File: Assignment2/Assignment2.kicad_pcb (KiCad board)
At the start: 2 copper layers, 51 parts, among them J1 USB_B_Micro, J2 Conn_01x02, J3 Conn_01x03, J4 Conn_01x02, SW1 SW_Push, U1 RP2040, U2 NCP1117-3.3_SOT223, U3 W25Q128JVS, U4 ABM8-272-T3, U5 MAX98357A, U6 VEML6040

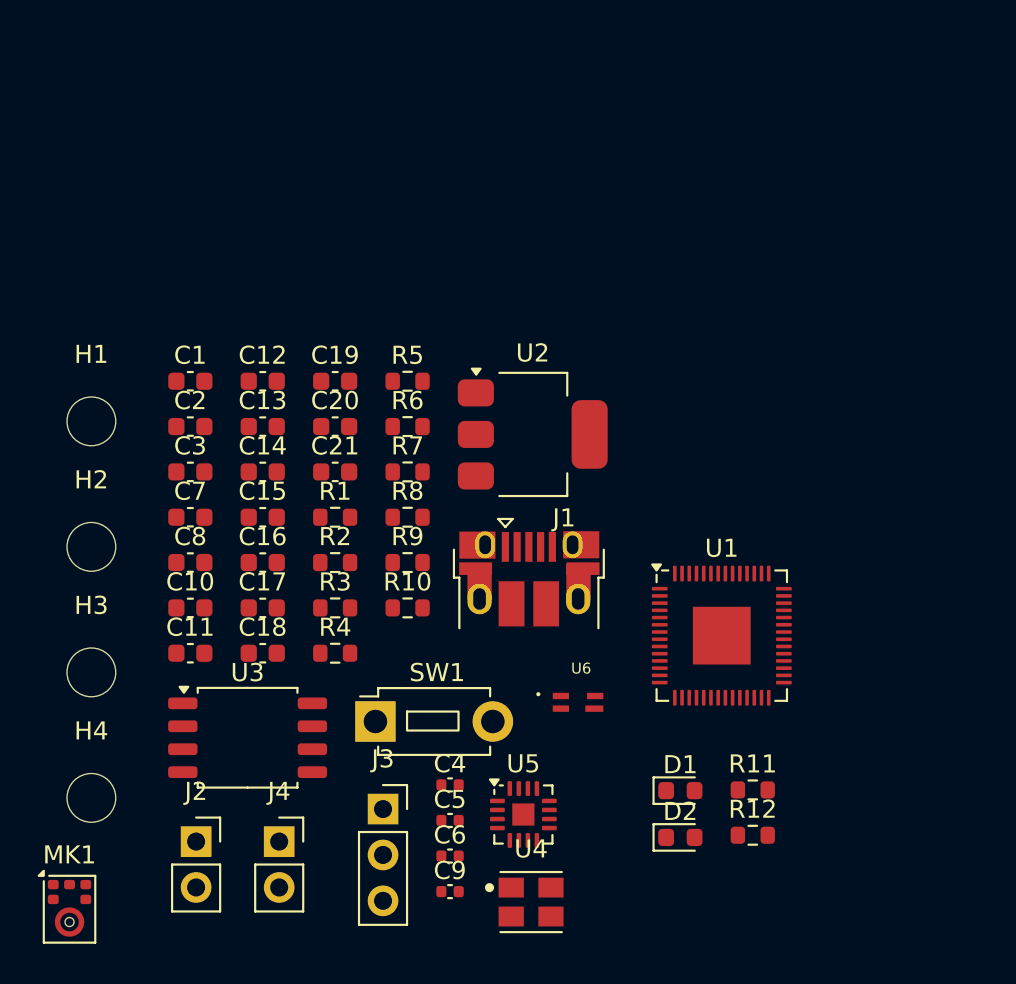
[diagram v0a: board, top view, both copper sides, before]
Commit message: route
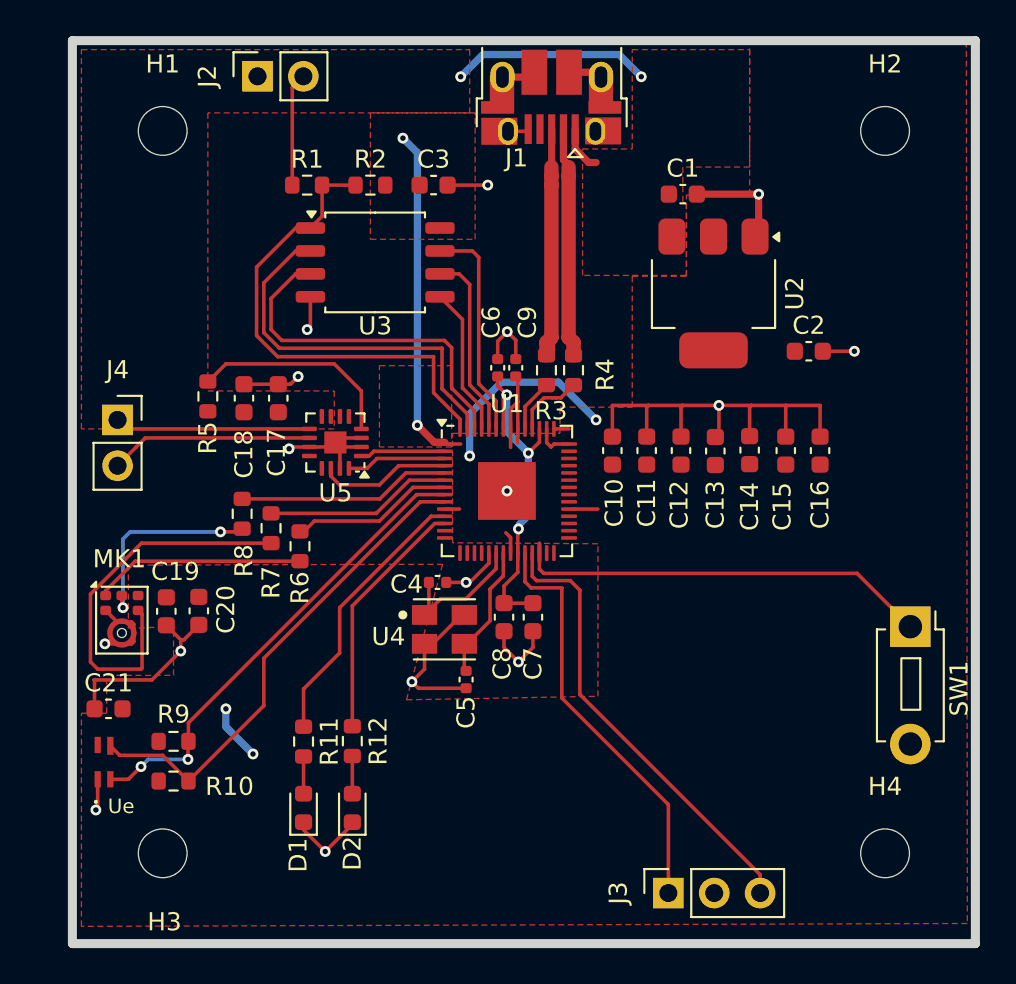
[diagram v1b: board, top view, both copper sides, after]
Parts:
- moved H2 49.6 mm to (145.0, 55.0)
- moved H4 44.1 mm to (145.0, 95.0)
- moved J2 42.5 mm to (110.2, 52.0), turned to 90 degrees
- moved C2 34.5 mm to (140.8, 67.2)
- moved C16 31.5 mm to (141.4, 72.7), turned to 90 degrees
- moved SW1 30.1 mm to (146.4, 82.5), turned to -90 degrees
- moved C9 29.2 mm to (124.5, 68.1), turned to 90 degrees
- moved C15 29.2 mm to (139.5, 72.7), turned to 90 degrees
- moved C1 29.2 mm to (133.8, 58.5)
- moved C11 27.6 mm to (131.8, 72.7), turned to 90 degrees
- moved U3 27.3 mm to (116.8, 62.3)
- moved C6 27.2 mm to (123.5, 68.1), turned to 90 degrees
- moved C14 27.0 mm to (137.5, 72.7), turned to 90 degrees
- moved J1 26.7 mm to (126.5, 53.1), turned to 180 degrees
- moved Ue 26.5 mm to (101.8, 90.0), turned to 90 degrees
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- renumbered U6 to Ue
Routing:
- net GND: track 0.00 -> 92.3 mm, vias 0 -> 16
- net +3.3V: track 0.00 -> 46.0 mm, vias 0 -> 6
- net /GPIO7: track 0.00 -> 27.3 mm
- net /QSPI_SS: track 0.00 -> 27.1 mm
- net /GPIO6: track 0.00 -> 26.2 mm, vias 0 -> 2
- net /SWD: track 0.00 -> 25.1 mm
- net /RUN: track 0.00 -> 24.3 mm
- net /USB_D+: track 0.00 -> 23.2 mm
- net /SWCLK: track 0.00 -> 23.1 mm
- net /QSPI_SD1: track 0.00 -> 21.3 mm
- net Net-(MK1-BCLK): track 0.00 -> 21.3 mm
- net /QSPI_SD2: track 0.00 -> 19.9 mm
- net +1V1: track 0.00 -> 19.1 mm, vias 0 -> 3
- net /GPIO8: track 0.00 -> 15.3 mm
- net /GPIO9: track 0.00 -> 13.7 mm
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- added copper zone on F.Cu, net +3.3V
- added copper zone on F.Cu, net +5V
- added copper zone on B.Cu, net GND
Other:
- board outline added: 50 x 50 mm
